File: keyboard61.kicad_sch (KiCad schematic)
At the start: 124 parts, among them SW1 Esc, SW10 9, SW11 0, SW12 -, SW13 =, SW14 Backspace, SW15 Tab, SW16 Q, SW17 W, SW18 E, SW19 R, SW2 1, SW20 T, SW21 Y, SW22 U, SW23 I, SW24 O, SW25 P, SW26 [, SW27 ], SW28 Backslash, SW29 Caps, SW3 2, SW30 A, SW31 S, SW32 D, SW33 F, SW34 G, SW35 H, SW36 J, SW37 K, SW38 L, SW39 ;, SW4 3, SW40 Quote, SW41 Enter, SW42 LShift, SW43 Z, SW44 X, SW45 C, SW46 V, SW47 B, SW48 N, SW49 M, SW5 4, SW50 ,, SW51 ., SW52 /, SW53 RShift, SW54 LCtrl, SW55 LWin, SW56 LAlt, SW57 Space, SW58 RAlt, SW59 Fn, SW6 5, SW60 Menu, SW61 RCtrl, SW62 RESET, SW7 6, SW8 7, SW9 8, U1 Raspberry Pi Pico

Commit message: BOM
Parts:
- SW15: footprint Button_Switch_Keyboard:SW_Cherry_MX_1.50u_PCB -> Keyboard61:SW_Cherry_MX_1.50u_PCB_SocketClearance
- SW16: footprint Button_Switch_Keyboard:SW_Cherry_MX_1.00u_PCB -> Keyboard61:SW_Cherry_MX_1.00u_PCB_SocketClearance
- U1: footprint Module:RaspberryPi_Pico_Common_THT -> Keyboard61:Pico_H_Bottom_Sockets_8_5mm

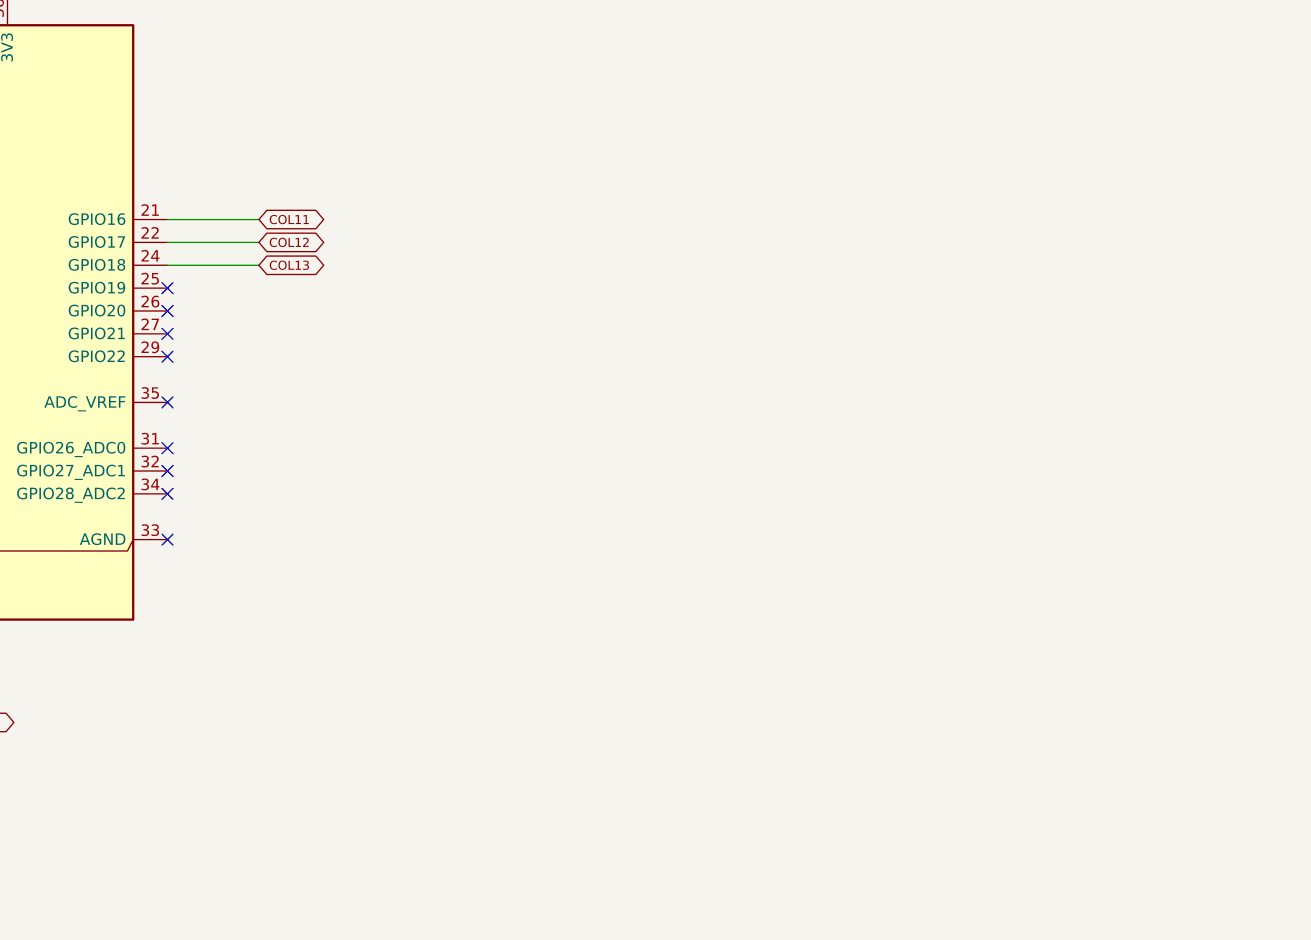
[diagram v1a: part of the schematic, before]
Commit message: BOM
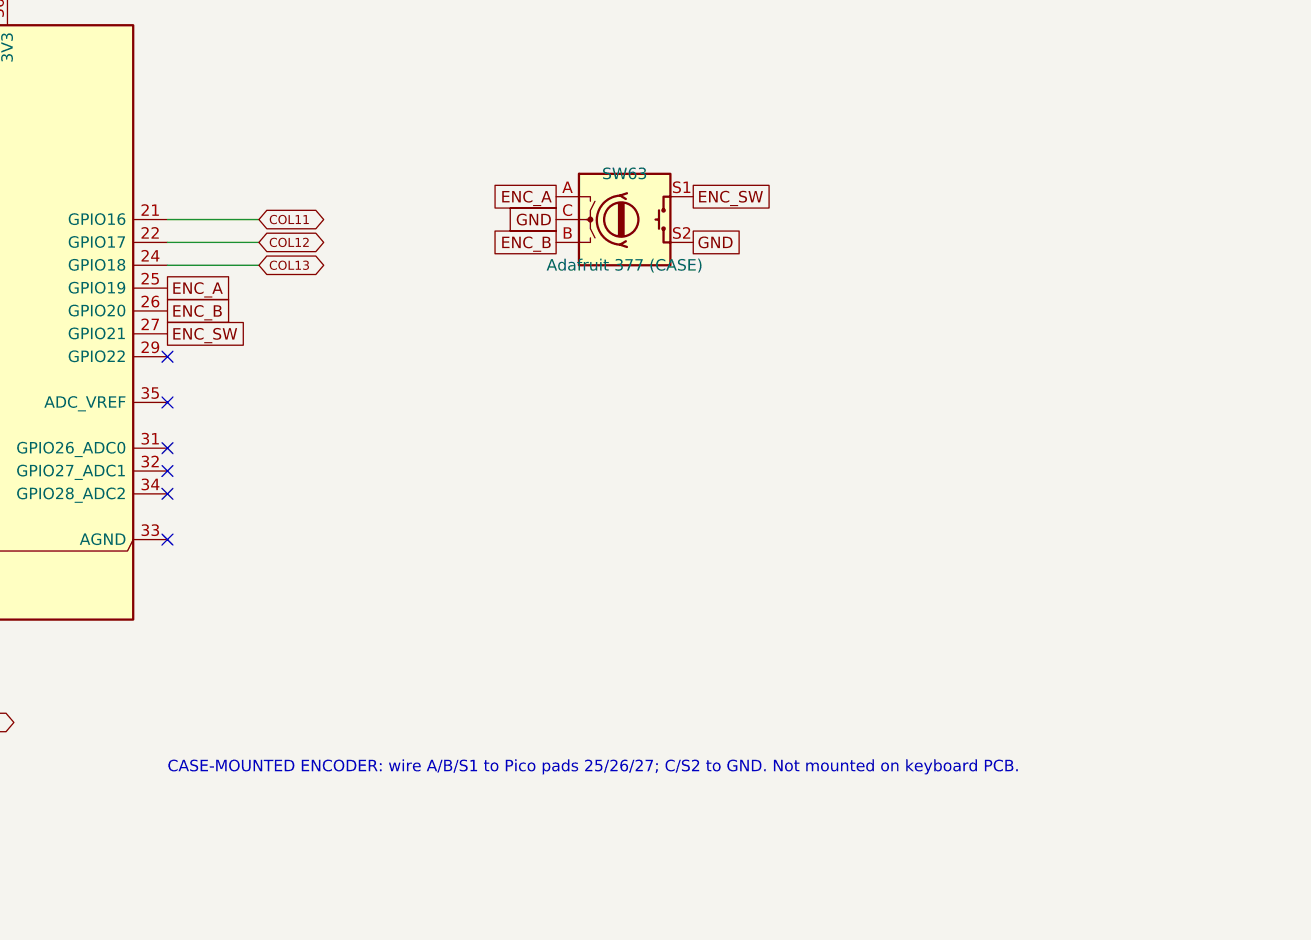
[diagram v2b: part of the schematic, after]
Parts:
- added SW63: Adafruit 377 (CASE), symbol Device:RotaryEncoder_Switch
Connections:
- net GND: now also SW63.C, SW63.S2
- net ENC_A: now reaches U1.25 (GPIO19)
- net ENC_A: now also SW63.A
- net ENC_B: now reaches U1.26 (GPIO20)
- net ENC_B: now also SW63.B
- net ENC_SW: now reaches U1.27 (GPIO21)
- net ENC_SW: now also SW63.S1
- no-connect marks 13 -> 10
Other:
- note added: "CASE-MOUNTED ENCODER: wire A/B/S1 to Pico pads 25/26/27; C/S2 to GND. Not mounted on keyboard PCB."
